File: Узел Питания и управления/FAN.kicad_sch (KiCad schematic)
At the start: 4 parts, among them M5 FAN_IN, M6 FAN_OUT

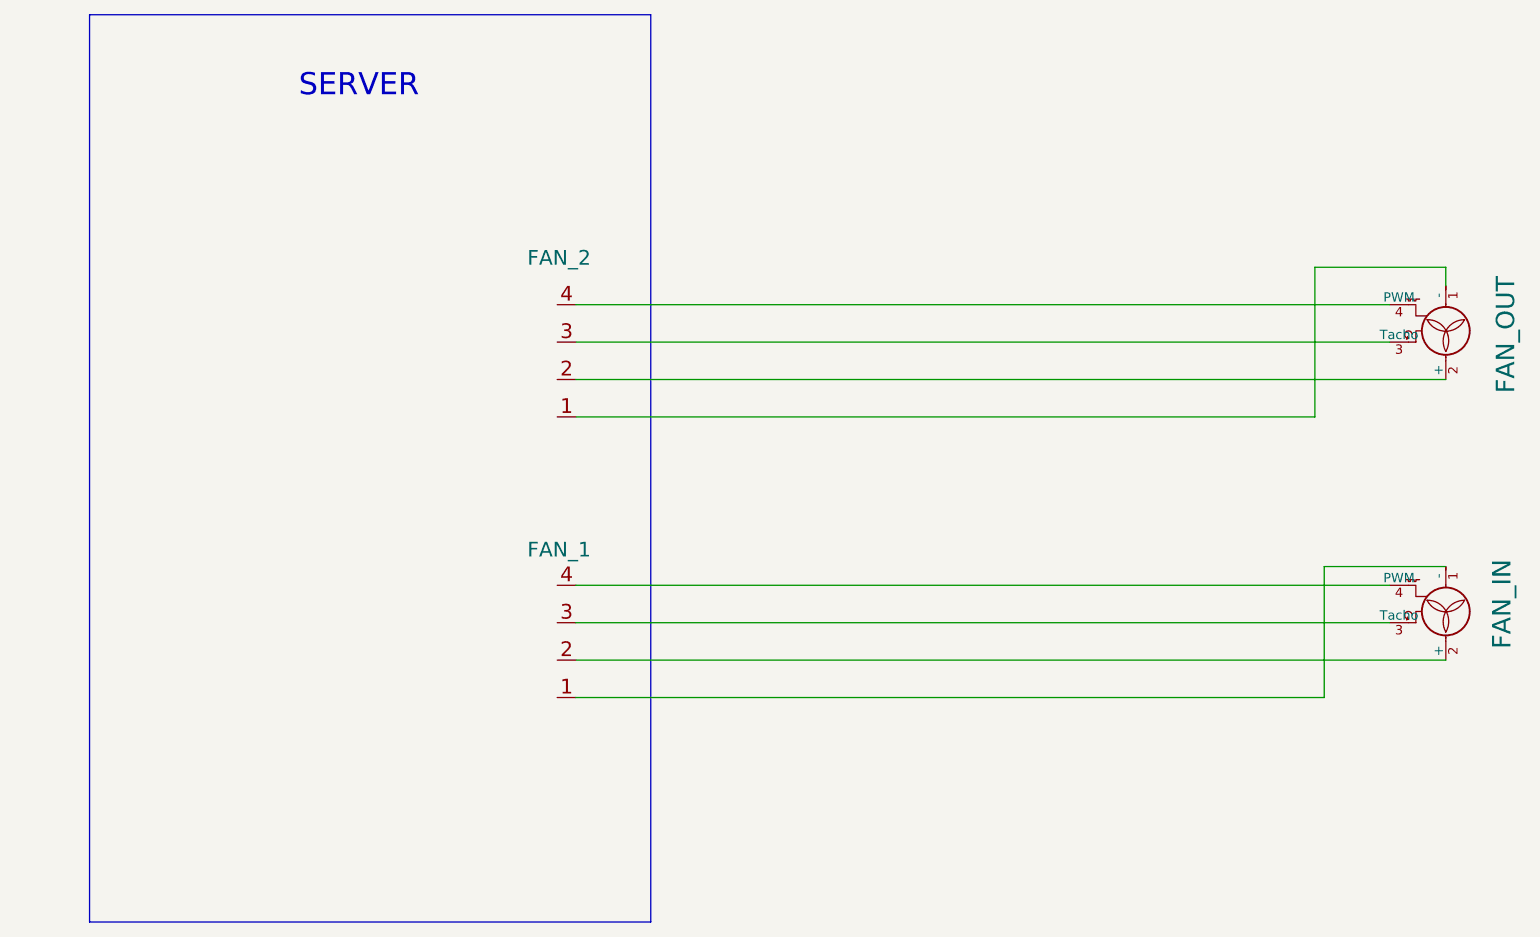
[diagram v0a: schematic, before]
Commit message: update schemas
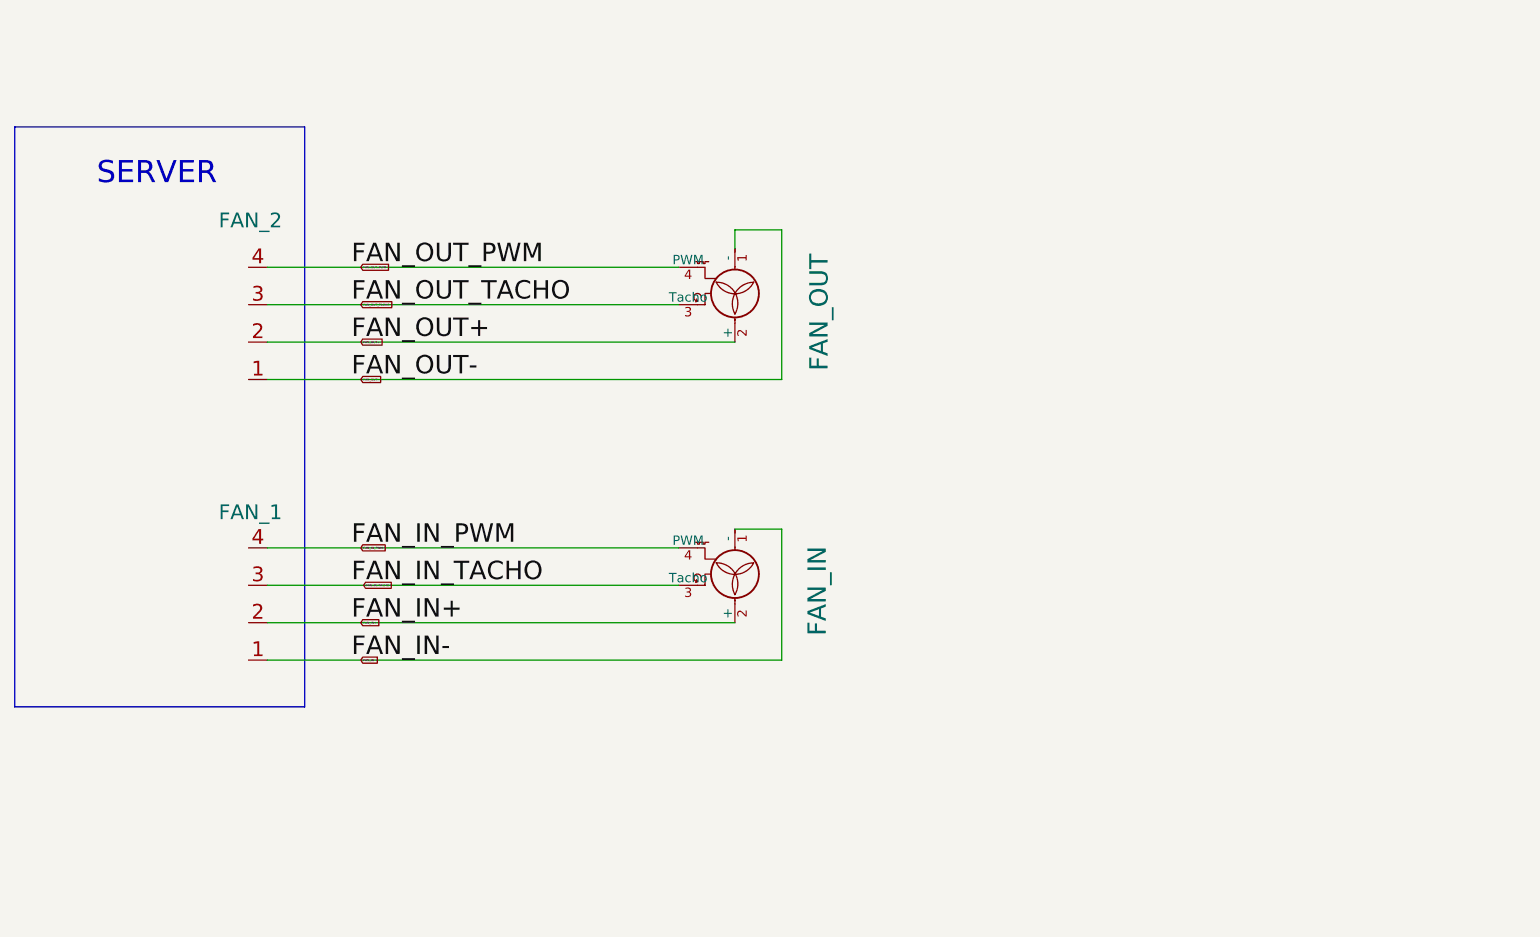
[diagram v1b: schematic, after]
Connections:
- net FAN_OUT-: now reaches FAN_2.1, M6.1 (-)
- net FAN_OUT+: now reaches FAN_2.2, M6.2 (+)
- net FAN_OUT_TACHO: now reaches FAN_2.3, M6.3 (Tacho)
- net FAN_OUT_PWM: now reaches FAN_2.4, M6.4 (PWM)
- net FAN_IN-: now reaches FAN_1.1, M5.1 (-)
- net FAN_IN+: now reaches FAN_1.2, M5.2 (+)
- net FAN_IN_TACHO: now reaches FAN_1.3, M5.3 (Tacho)
- net FAN_IN_PWM: now reaches FAN_1.4, M5.4 (PWM)
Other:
- moved on the sheet: FAN_1, FAN_2
